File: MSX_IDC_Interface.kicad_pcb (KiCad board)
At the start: 2 copper layers, 103 x 66 mm, 21 parts, among them J1 DE1 GPIO, Q1 2N2222, Q2 2N2222, U1 74LVC245A, U2 74LVC245A, U3 74LVC245A, U4 74LVC245A, U5 74LVC245A, U7 74LS00

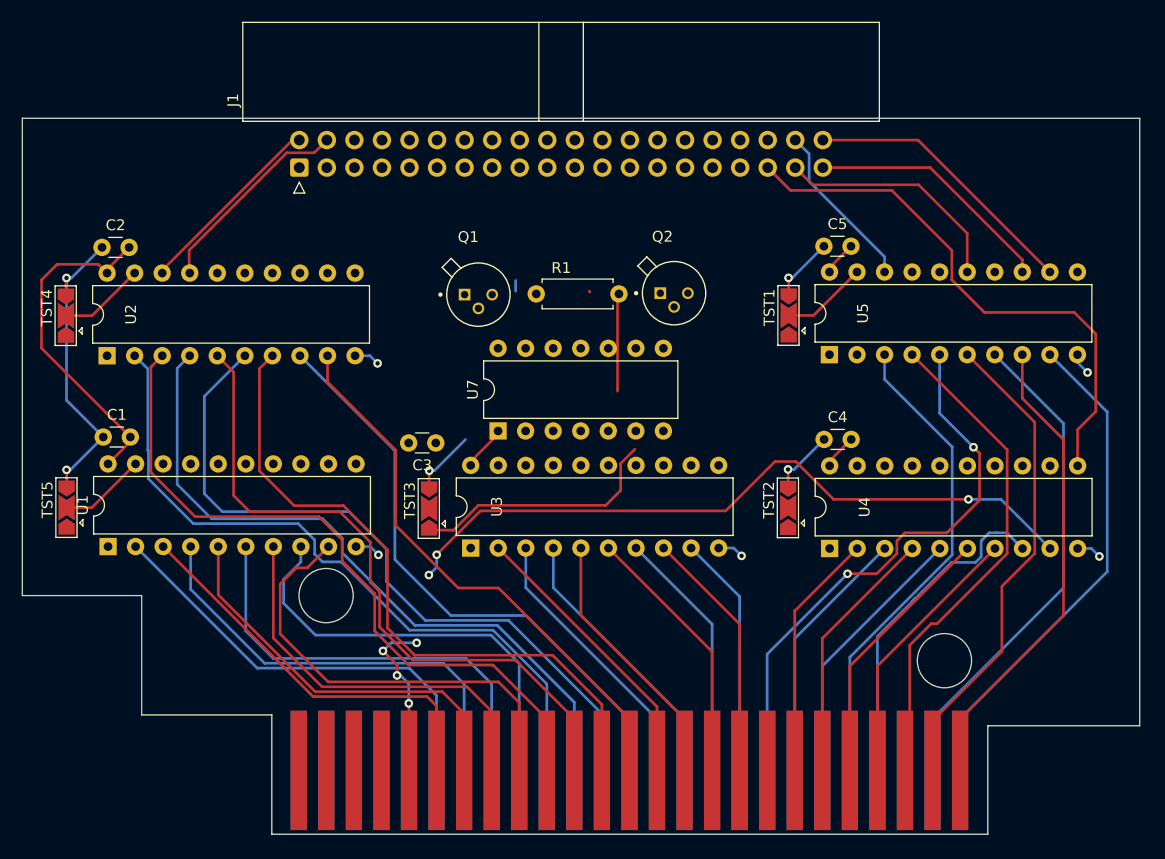
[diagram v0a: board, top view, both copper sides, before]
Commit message: Safe guard commit - progressing with routing
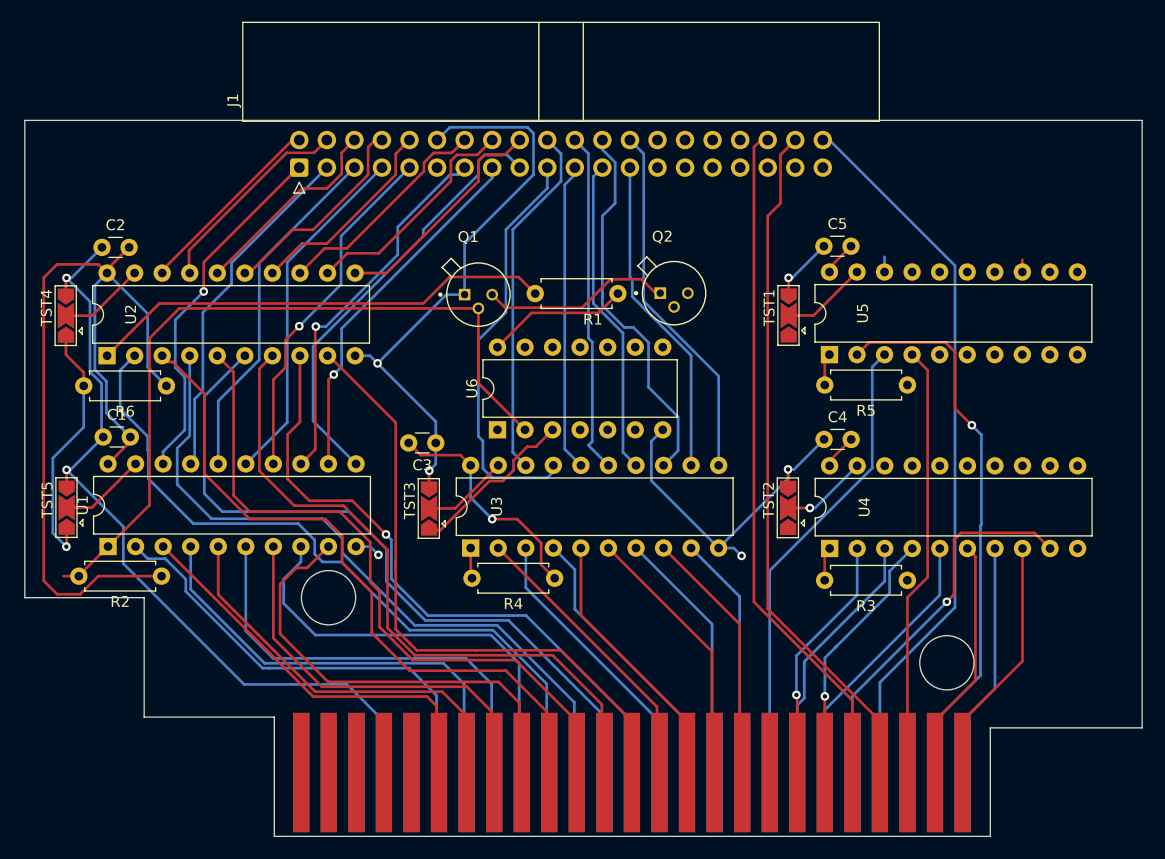
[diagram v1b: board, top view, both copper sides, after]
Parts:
- removed U7: 74LS00, Package_DIP:DIP-14_W7.62mm
- added R2: 1k, Resistor_THT:R_Axial_DIN0207_L6.3mm_D2.5mm_P7.62mm_Horizontal, F.Cu at (64.8, 62.4)
- added R3: 1k, Resistor_THT:R_Axial_DIN0207_L6.3mm_D2.5mm_P7.62mm_Horizontal, F.Cu at (133.5, 62.8)
- added R4: 1k, Resistor_THT:R_Axial_DIN0207_L6.3mm_D2.5mm_P7.62mm_Horizontal, F.Cu at (101.0, 62.6)
- added R5: 1k, Resistor_THT:R_Axial_DIN0207_L6.3mm_D2.5mm_P7.62mm_Horizontal, F.Cu at (133.5, 44.8)
- added R6: 1k, Resistor_THT:R_Axial_DIN0207_L6.3mm_D2.5mm_P7.62mm_Horizontal, F.Cu at (65.2, 44.9)
- added U6: 74LS00, Package_DIP:DIP-14_W7.62mm, F.Cu at (95.7, 48.9)
- moved R1 7.53 mm to (106.8, 36.4), turned to 180 degrees
- moved CONN1 0.30 mm to (101.8, 51.0)
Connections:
- J1 pad 11: +5V -> unconnected-(J1-Pad11)
- J1 pad 19: /C_BUSDIR -> C_A12
- J1 pad 21: /C_IORQ -> C_A7
- J1 pad 22: C_A12 -> C_A6
- J1 pad 23: /C_MREQ -> C_A10
- J1 pad 24: C_A7 -> C_A11
- J1 pad 25: /C_WR -> C_A15
- J1 pad 26: C_A6 -> C_A9
- J1 pad 28: C_A10 -> /C_WR
- J1 pad 29: +3.3V -> unconnected-(J1-Pad29)
- J1 pad 31: /C_RESET -> /C_MREQ
- J1 pad 32: C_A11 -> /C_IORQ
- J1 pad 33: C_CLOCK -> /C_SLTSL
- J1 pad 34: C_A15 -> /C_CS1
- J1 pad 35: C_SOUNDIN -> /C_CS2
- J1 pad 36: C_A9 -> /BUSDIR
- J1 pad 37: /C_SLTSL -> /C_M1
- J1 pad 38: /C_CS1 -> /INT
- J1 pad 39: /C_WAIT -> C_CLOCK
- J1 pad 40: /C_INT -> /WAIT
- R1 pad 2: Net-(Q2-Pad3) -> Net-(R1-Pad2)
- U1 pad 1: unconnected-(U1-Pad1) -> /RD
- U2 pad 1: unconnected-(U2-Pad1) -> Net-(R1-Pad2)
- U3 pad 1: unconnected-(U3-Pad1) -> Net-(R4-Pad2)
- U4 pad 1: unconnected-(U4-Pad1) -> Net-(R3-Pad2)
- U4 pad 11: C_CLOCK -> /C_M1
- U4 pad 12: /C_WAIT -> /C_CS2
- U4 pad 13: /C_INT -> /C_CS1
- U4 pad 14: /C_BUSDIR -> /C_SLTSL
- U4 pad 6: /BUSDIR -> /SLTSL
- U4 pad 7: /INT -> /CS1
- U4 pad 8: /WAIT -> /CS2
- U4 pad 9: /RESET -> /M1
- U5 pad 1: unconnected-(U5-Pad1) -> Net-(R5-Pad2)
- U5 pad 11: /C_CS1 -> unconnected-(U5-Pad11)
- U5 pad 12: /C_CS2 -> unconnected-(U5-Pad12)
- U5 pad 13: /C_CS12 -> unconnected-(U5-Pad13)
- U5 pad 14: /C_SLTSL -> unconnected-(U5-Pad14)
- U5 pad 15: /C_RESET -> C_CLOCK
- U5 pad 17: /C_M1 -> /C_RESET
- U5 pad 18: C_SOUNDIN -> /C_CS12
- U5 pad 2: SOUNDIN -> /CS12
- U5 pad 3: /M1 -> /RESET
- U5 pad 6: /SLTSL -> unconnected-(U5-Pad6)
- U5 pad 7: /CS12 -> unconnected-(U5-Pad7)
- U5 pad 8: /CS2 -> unconnected-(U5-Pad8)
- U5 pad 9: /CS1 -> unconnected-(U5-Pad9)
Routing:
- net GNDREF: track 58.6 -> 167.9 mm, vias 10 -> 8
- net +3.3V: track 37.8 -> 124.3 mm, vias 0 -> 1
- net /RD: track 22.8 -> 93.5 mm, vias 0 -> 1
- net CLOCK: track 67.4 -> 0.00 mm, vias 6 -> 0
- net C_CLOCK: track 51.0 -> 0.00 mm
- net Net-(R1-Pad2): track 0.00 -> 43.1 mm
- net C_D0: track 0.00 -> 40.4 mm
- net /INT: track 24.9 -> 63.6 mm
- net C_A12: track 0.00 -> 38.2 mm
- net /BUSDIR: track 24.9 -> 62.9 mm
- net C_A11: track 0.00 -> 35.4 mm
- net /WAIT: track 31.6 -> 66.6 mm
- net C_D2: track 0.00 -> 34.5 mm, vias 0 -> 1
- net C_D1: track 0.00 -> 33.6 mm, vias 0 -> 1
- net C_A9: track 0.00 -> 33.4 mm
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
